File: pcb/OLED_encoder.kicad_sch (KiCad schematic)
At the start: 19 parts, among them J1 Conn_01x10, J2 Conn_02x08_Odd_Even, U1 ACZ11BR1E-20FD1-20C

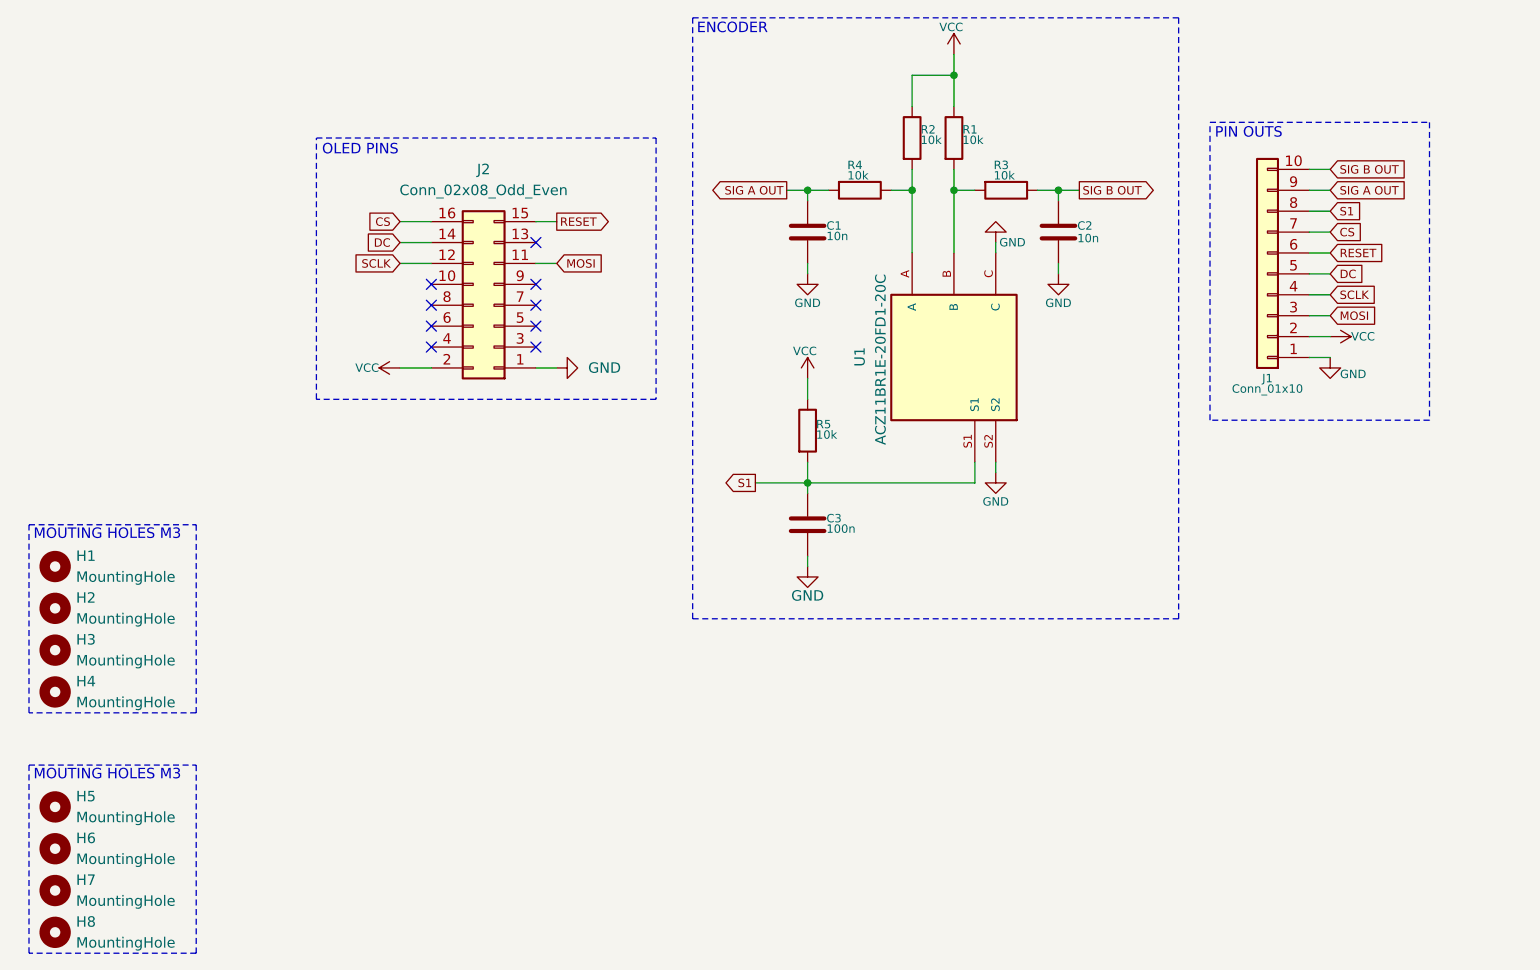
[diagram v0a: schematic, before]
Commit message: refactor
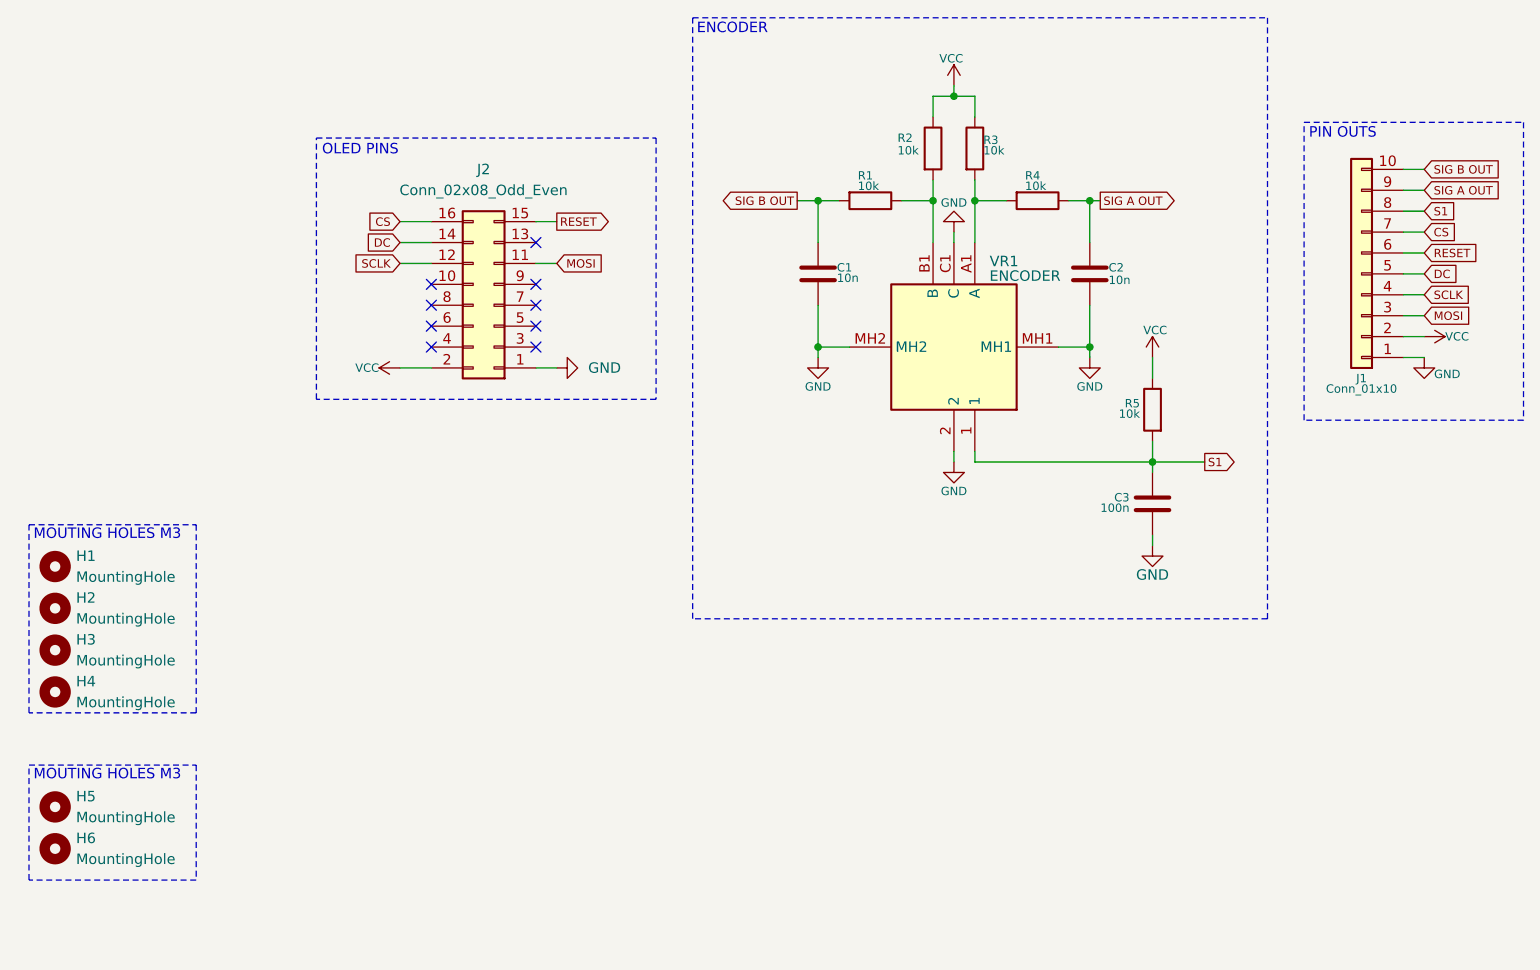
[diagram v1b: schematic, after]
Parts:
- removed H7, H8: MountingHole, MountingHole:MountingHole_3.5mm, symbol Mechanical:MountingHole
- removed U1: ACZ11BR1E-20FD1-20C, ACZ11BR1E-20FD1-20C:CUI_ACZ11BR1E-20FD1-20C, symbol ACZ11BR1E-20FD1-20C:ACZ11BR1E-20FD1-20C
- added VR1: ENCODER, PEC11R4220FS0024, symbol PEC11R-4220F-S0024:PEC11R-4220F-S0024
- H5, H6: footprint MountingHole:MountingHole_3.5mm -> MountingHole:MountingHole_3.2mm_M3
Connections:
- net GND: now also VR1.2, VR1.C1 (C), VR1.MH1, VR1.MH2
- net S1: now also VR1.1
- net SIG A OUT: now also C2.1, R4.1; no longer C1.1, R4.2
- net SIG B OUT: now also C1.1, R1.2; no longer C2.1, R3.1
- net VCC: now also R3.1; no longer R1.1
- net at R2.2: now also R1.1, VR1.B1 (B); no longer R4.1
- net at R3.2: now also R4.2, VR1.A1 (A); no longer R1.2
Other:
- moved on the sheet: J1
